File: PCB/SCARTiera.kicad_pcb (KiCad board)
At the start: 2 copper layers, 214 x 123 mm, 25 parts, among them J1 SCART-F, J2 SCART-F, J3 SCART-F, J4 SCART-TV, J5 SCART-F, J6 SCART-F, J7 SCART-F, SW1 SW_DIP_x09, SW2 SW_DIP_x09, SW3 SW_DIP_x09, SW4 SW_DIP_x09, SW5 SW_DIP_x09, SW6 SW_DIP_x09

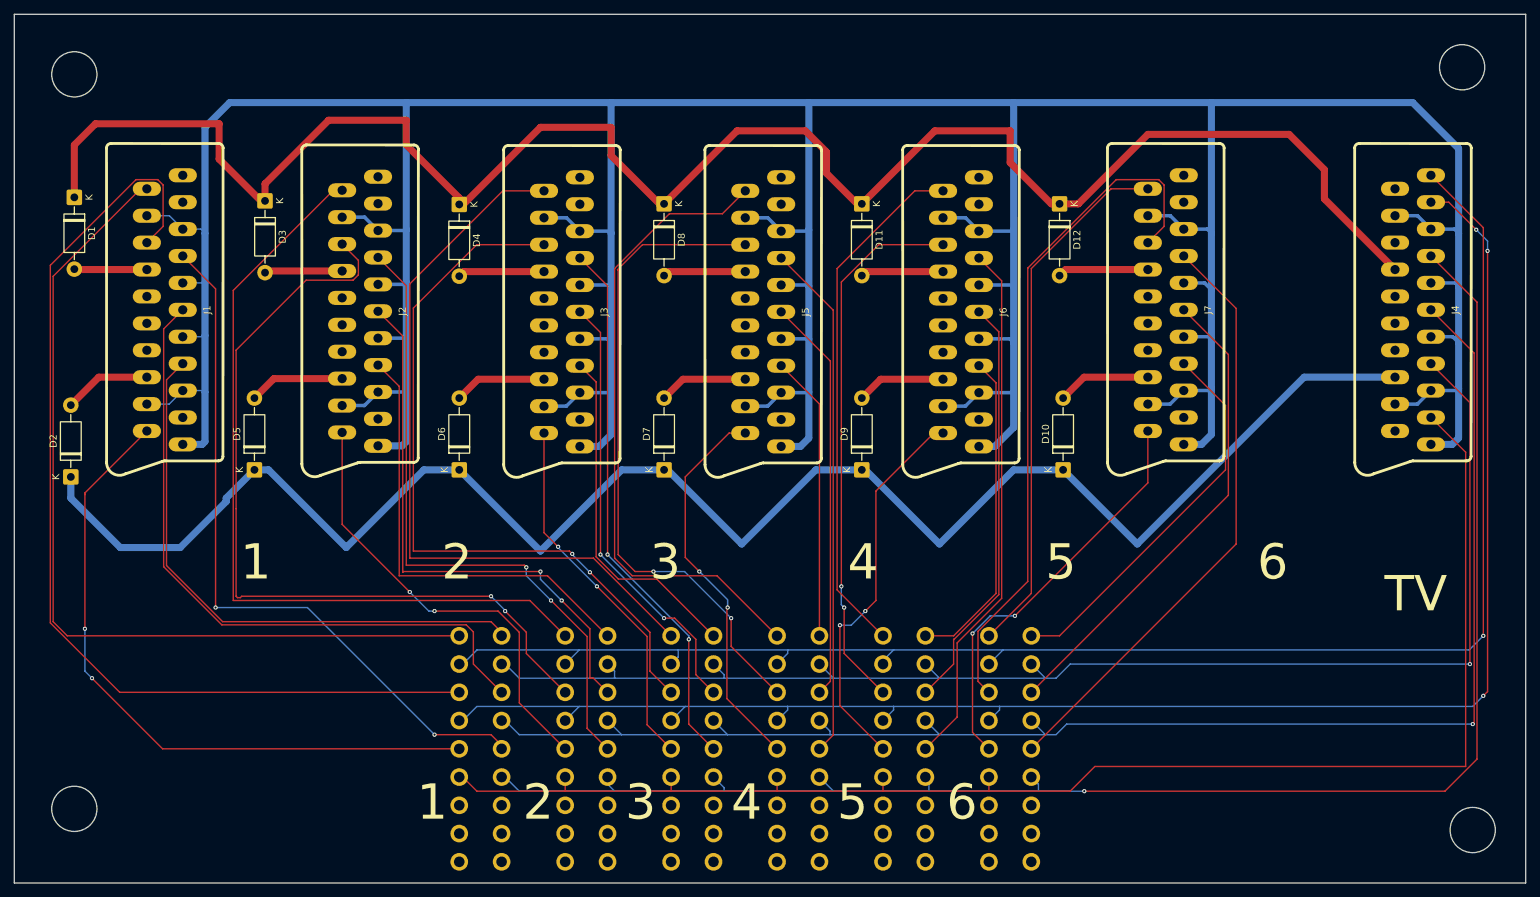
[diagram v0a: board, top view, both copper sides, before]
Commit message: Add files via upload
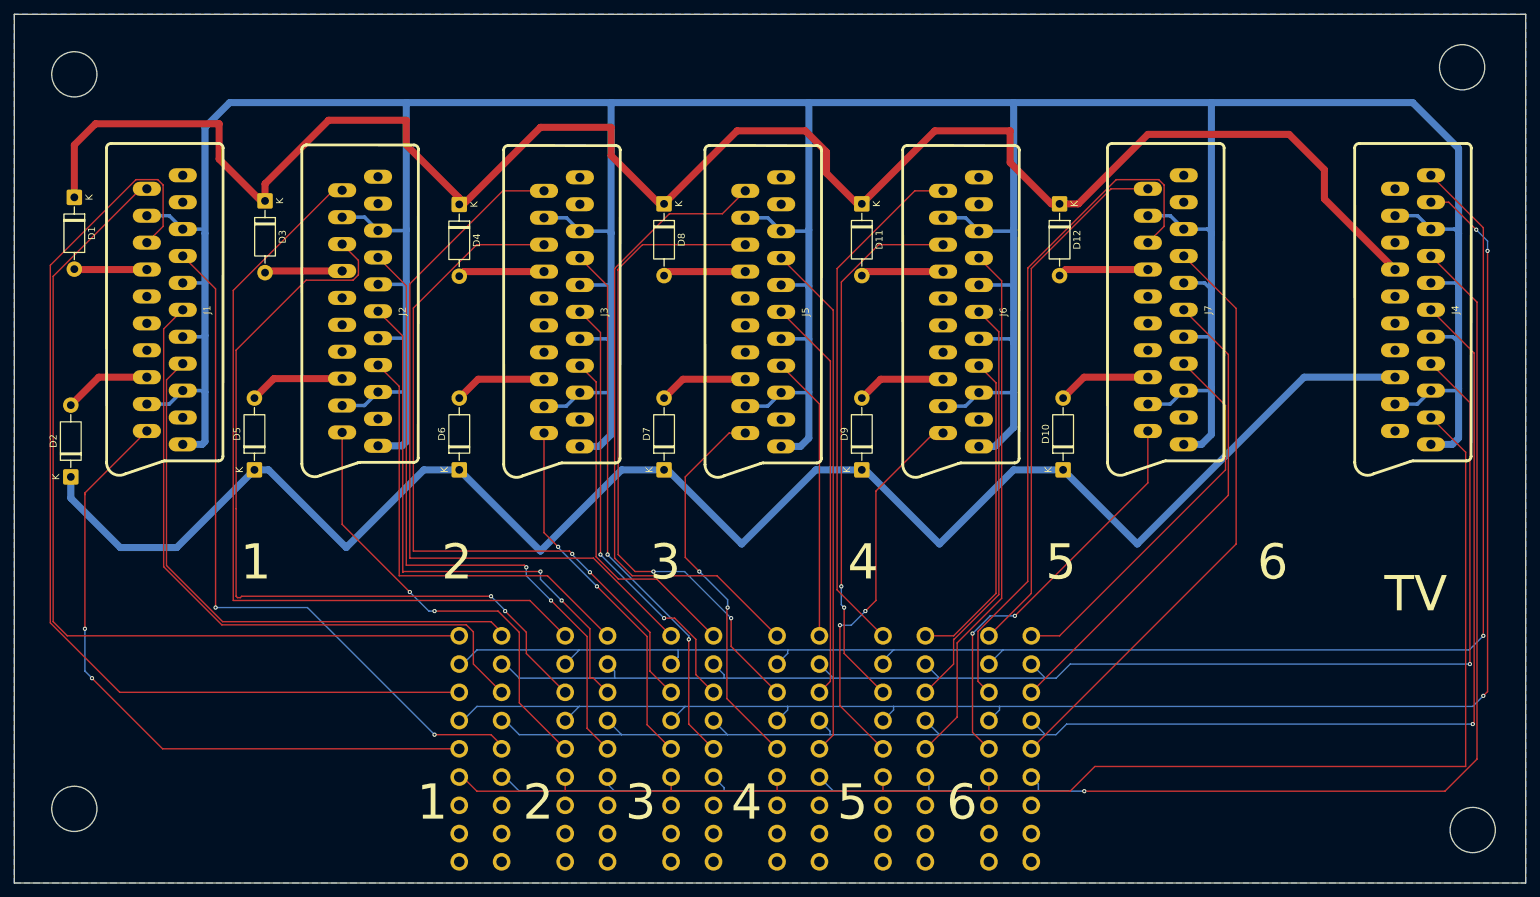
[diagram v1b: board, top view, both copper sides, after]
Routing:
- added copper zone on B.Cu, net GND
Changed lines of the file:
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@@
 			(pinfunction "P4")
 			(pintype "passive")
+			(zone_connect 2)
 		)
 		(pad "5" thru_hole oval
@@
 			(pinfunction "P5")
 			(pintype "passive")
+			(zone_connect 2)
 		)
 		(pad "6" thru_hole oval
@@
 			(pinfunction "P9")
 			(pintype "passive")
+			(zone_connect 2)
 		)
 		(pad "10" thru_hole oval
@@
 			(pinfunction "P13")
 			(pintype "passive")
+			(zone_connect 2)
 		)
 		(pad "14" thru_hole oval
@@
 			(pinfunction "P17")
 			(pintype "passive")
+			(zone_connect 2)
 		)
 		(pad "18" thru_hole oval
@@
 			(pinfunction "P18")
 			(pintype "passive")
+			(zone_connect 2)
 		)
 		(pad "19" thru_hole oval
@@
 			(pinfunction "P21")
 			(pintype "passive")
+			(zone_connect 2)
 		)
 		(embedded_fonts no)
@@
 			(pinfunction "P4")
 			(pintype "passive")
+			(zone_connect 2)
 		)
 		(pad "5" thru_hole oval
@@
 			(pinfunction "P5")
 			(pintype "passive")
+			(zone_connect 2)
 		)
 		(pad "6" thru_hole oval
@@
 			(pinfunction "P9")
 			(pintype "passive")
+			(zone_connect 2)
 		)
 		(pad "10" thru_hole oval
@@
 			(pinfunction "P13")
 			(pintype "passive")
+			(zone_connect 2)
 		)
 		(pad "14" thru_hole oval
@@
 			(pinfunction "P17")
 			(pintype "passive")
+			(zone_connect 2)
 		)
 		(pad "18" thru_hole oval
@@
 			(pinfunction "P18")
 			(pintype "passive")
+			(zone_connect 2)
 		)
 		(pad "19" thru_hole oval
@@
 			(pinfunction "P21")
 			(pintype "passive")
+			(zone_connect 2)
 		)
 		(embedded_fonts no)
@@
 			(pinfunction "P4")
 			(pintype "passive")
+			(zone_connect 2)
 		)
 		(pad "5" thru_hole oval
@@
 			(pinfunction "P5")
 			(pintype "passive")
+			(zone_connect 2)
 		)
 		(pad "6" thru_hole oval
@@
 			(pinfunction "P9")
 			(pintype "passive")
+			(zone_connect 2)
 		)
 		(pad "10" thru_hole oval
@@
 			(pinfunction "P13")
 			(pintype "passive")
+			(zone_connect 2)
 		)
 		(pad "14" thru_hole oval
@@
 			(pinfunction "P17")
 			(pintype "passive")
+			(zone_connect 2)
 		)
 		(pad "18" thru_hole oval
@@
 			(pinfunction "P18")
 			(pintype "passive")
+			(zone_connect 2)
 		)
 		(pad "19" thru_hole oval
@@
 			(pinfunction "P21")
 			(pintype "passive")
+			(zone_connect 2)
 		)
 		(embedded_fonts no)
@@
 			(pinfunction "P4")
 			(pintype "passive")
+			(zone_connect 2)
 		)
 		(pad "5" thru_hole oval
@@
 			(pinfunction "P5")
 			(pintype "passive")
+			(zone_connect 2)
 		)
 		(pad "6" thru_hole oval
@@
 			(pinfunction "P9")
 			(pintype "passive")
+			(zone_connect 2)
 		)
 		(pad "10" thru_hole oval
@@
 			(pinfunction "P13")
 			(pintype "passive")
+			(zone_connect 2)
 		)
 		(pad "14" thru_hole oval
@@
 			(pinfunction "P17")
 			(pintype "passive")
+			(zone_connect 2)
 		)
 		(pad "18" thru_hole oval
@@
 			(pinfunction "P18")
 			(pintype "passive")
+			(zone_connect 2)
 		)
 		(pad "19" thru_hole oval
@@
 			(pinfunction "P21")
 			(pintype "passive")
+			(zone_connect 2)
 		)
 		(embedded_fonts no)
@@
 			(pinfunction "P4")
 			(pintype "passive")
+			(zone_connect 2)
 		)
 		(pad "5" thru_hole oval
@@
 			(pinfunction "P5")
 			(pintype "passive")
+			(zone_connect 2)
 		)
 		(pad "6" thru_hole oval
@@
 			(pinfunction "P9")
 			(pintype "passive")
+			(zone_connect 2)
 		)
 		(pad "10" thru_hole oval
@@
 			(pinfunction "P13")
 			(pintype "passive")
+			(zone_connect 2)
 		)
 		(pad "14" thru_hole oval
@@
 			(pinfunction "P17")
 			(pintype "passive")
+			(zone_connect 2)
 		)
 		(pad "18" thru_hole oval
@@
 			(pinfunction "P18")
 			(pintype "passive")
+			(zone_connect 2)
 		)
 		(pad "19" thru_hole oval
@@
 			(pinfunction "P21")
 			(pintype "passive")
+			(zone_connect 2)
 		)
 		(embedded_fonts no)
@@
 			(pinfunction "P4")
 			(pintype "passive")
+			(zone_connect 2)
 		)
 		(pad "5" thru_hole oval
@@
 			(pinfunction "P5")
 			(pintype "passive")
+			(zone_connect 2)
 		)
 		(pad "6" thru_hole oval
@@
 			(pinfunction "P9")
 			(pintype "passive")
+			(zone_connect 2)
 		)
 		(pad "10" thru_hole oval
@@
 			(pinfunction "P13")
 			(pintype "passive")
+			(zone_connect 2)
 		)
 		(pad "14" thru_hole oval
@@
 			(pinfunction "P17")
 			(pintype "passive")
+			(zone_connect 2)
 		)
 		(pad "18" thru_hole oval
@@
 			(pinfunction "P18")
 			(pintype "passive")
+			(zone_connect 2)
 		)
 		(pad "19" thru_hole oval
@@
 			(pinfunction "P21")
 			(pintype "passive")
+			(zone_connect 2)
 		)
 		(embedded_fonts no)
@@
 			(pinfunction "P4")
 			(pintype "passive")
+			(zone_connect 2)
 		)
 		(pad "5" thru_hole oval
@@
 			(pinfunction "P5")
 			(pintype "passive")
+			(zone_connect 2)
 		)
 		(pad "6" thru_hole oval
@@
 			(pinfunction "P9")
 			(pintype "passive")
+			(zone_connect 2)
 		)
 		(pad "10" thru_hole oval
@@
 			(pinfunction "P13")
 			(pintype "passive")
+			(zone_connect 2)
 		)
 		(pad "14" thru_hole oval
@@
 			(pinfunction "P17")
 			(pintype "passive")
+			(zone_connect 2)
 		)
 		(pad "18" thru_hole oval
@@
 			(pinfunction "P18")
 			(pintype "passive")
+			(zone_connect 2)
 		)
 		(pad "19" thru_hole oval
@@
 			(pinfunction "P21")
 			(pintype "passive")
+			(zone_connect 2)
 		)
 		(embedded_fonts no)
@@
 	)
 	(segment
-		(start 36 122)
-		(end 44.5 122)
-		(width 1)
-		(layer "B.Cu")
-		(net 3)
-	)
-	(segment
 		(start 113 111)
 		(end 113.5 111)
@@
 	)
 	(segment
-		(start 51 115.5)
-		(end 51 115)
-		(width 1)
-		(layer "B.Cu")
-		(net 3)
-	)
-	(segment
-		(start 51 115)
-		(end 55 111)
+		(start 36 122)
+		(end 44 122)
 		(width 1)
 		(layer "B.Cu")
@@
 	)
 	(segment
+		(start 29 115)
+		(end 36 122)
+		(width 1)
+		(layer "B.Cu")
+		(net 3)
+	)
+	(segment
 		(start 107 111)
 		(end 113 111)
@@
 	)
 	(segment
-		(start 79 111)
-		(end 84 111)
+		(start 44 122)
+		(end 55 111)
 		(width 1)
 		(layer "B.Cu")
@@
 	)
 	(segment
-		(start 203.62 97.88)
-		(end 216.5 97.88)
+		(start 29 112)
+		(end 29 115)
 		(width 1)
 		(layer "B.Cu")
@@
 	)
 	(segment
-		(start 141.5 111)
-		(end 152 121.5)
+		(start 79 111)
+		(end 84 111)
 		(width 1)
 		(layer "B.Cu")
@@
 	)
 	(segment
-		(start 29 112)
-		(end 29 115)
+		(start 203.62 97.88)
+		(end 216.5 97.88)
 		(width 1)
 		(layer "B.Cu")
@@
 	)
 	(segment
-		(start 134.5 111)
-		(end 141 111)
+		(start 141.5 111)
+		(end 152 121.5)
 		(width 1)
 		(layer "B.Cu")
@@
 	)
 	(segment
-		(start 44.5 122)
-		(end 51 115.5)
+		(start 134.5 111)
+		(end 141 111)
 		(width 1)
 		(layer "B.Cu")
@@
 	)
 	(segment
-		(start 29 115)
-		(end 36 122)
-		(width 1)
-		(layer "B.Cu")
-		(net 3)
-	)
-	(segment
 		(start 141 111)
 		(end 141.5 111)
@@
 		(start 39.77 75.02)
 		(end 42.955 75.02)
-		(width 0.2)
+		(width 0.5)
 		(layer "B.Cu")
 		(net 9)
@@
 		(start 44.85 76.915)
 		(end 47.415 76.915)
-		(width 0.2)
+		(width 0.5)
 		(layer "B.Cu")
 		(net 9)
@@
 		(start 44.85 92.155)
 		(end 47.845 92.155)
-		(width 0.2)
+		(width 0.5)
 		(layer "B.Cu")
 		(net 9)
@@
 		(start 44.85 84.535)
 		(end 47.965 84.535)
-		(width 0.2)
+		(width 0.5)
 		(layer "B.Cu")
 		(net 9)
@@
 		(start 39.77 101.69)
 		(end 42.935 101.69)
-		(width 0.2)
+		(width 0.5)
 		(layer "B.Cu")
 		(net 9)
@@
 		(start 42.935 101.69)
 		(end 44.85 99.775)
-		(width 0.2)
+		(width 0.5)
 		(layer "B.Cu")
 		(net 9)
@@
 		(start 42.955 75.02)
 		(end 44.85 76.915)
-		(width 0.2)
+		(width 0.5)
 		(layer "B.Cu")
 		(net 9)
@@
 		(start 44.85 99.775)
 		(end 47.775 99.775)
-		(width 0.2)
+		(width 0.5)
 		(layer "B.Cu")
 		(net 9)
@@
 		(net 99)
 	)
+	(zone
+		(net 9)
+		(net_name "GND")
+		(layer "B.Cu")
+		(hatch edge 0.5)
+		(connect_pads
+			(clearance 0.5)
+		)
+		(min_thickness 0.25)
+		(filled_areas_thickness no)
+		(fill yes
+			(thermal_gap 0.5)
+			(thermal_bridge_width 0.5)
+		)
+		(polygon
+			(pts
+				(xy 21 46.5) (xy 21 169.5) (xy 235 169.5) (xy 235 46.5)
+			)
+		)
+	)
 	(embedded_fonts no)
